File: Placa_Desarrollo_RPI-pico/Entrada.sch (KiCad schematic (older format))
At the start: 24 parts, among them J10 Conn_01x03_Female, J11 Conn_01x03_Female, J9 Conn_01x03_Female, SW2 SW_Push, SW3 Rotary_Encoder_Switch, SW4 SW_Push, SW5 SW_Push

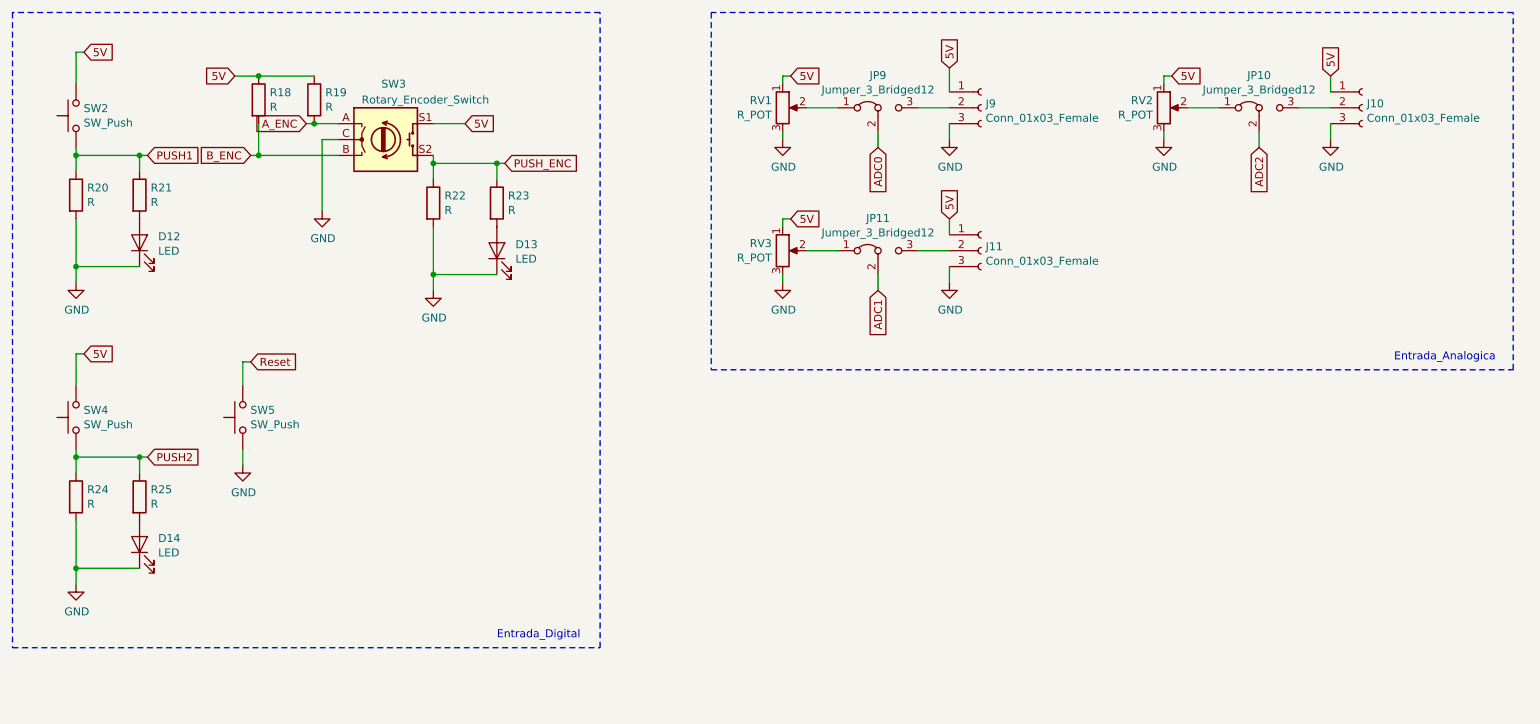
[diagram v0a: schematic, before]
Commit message: -
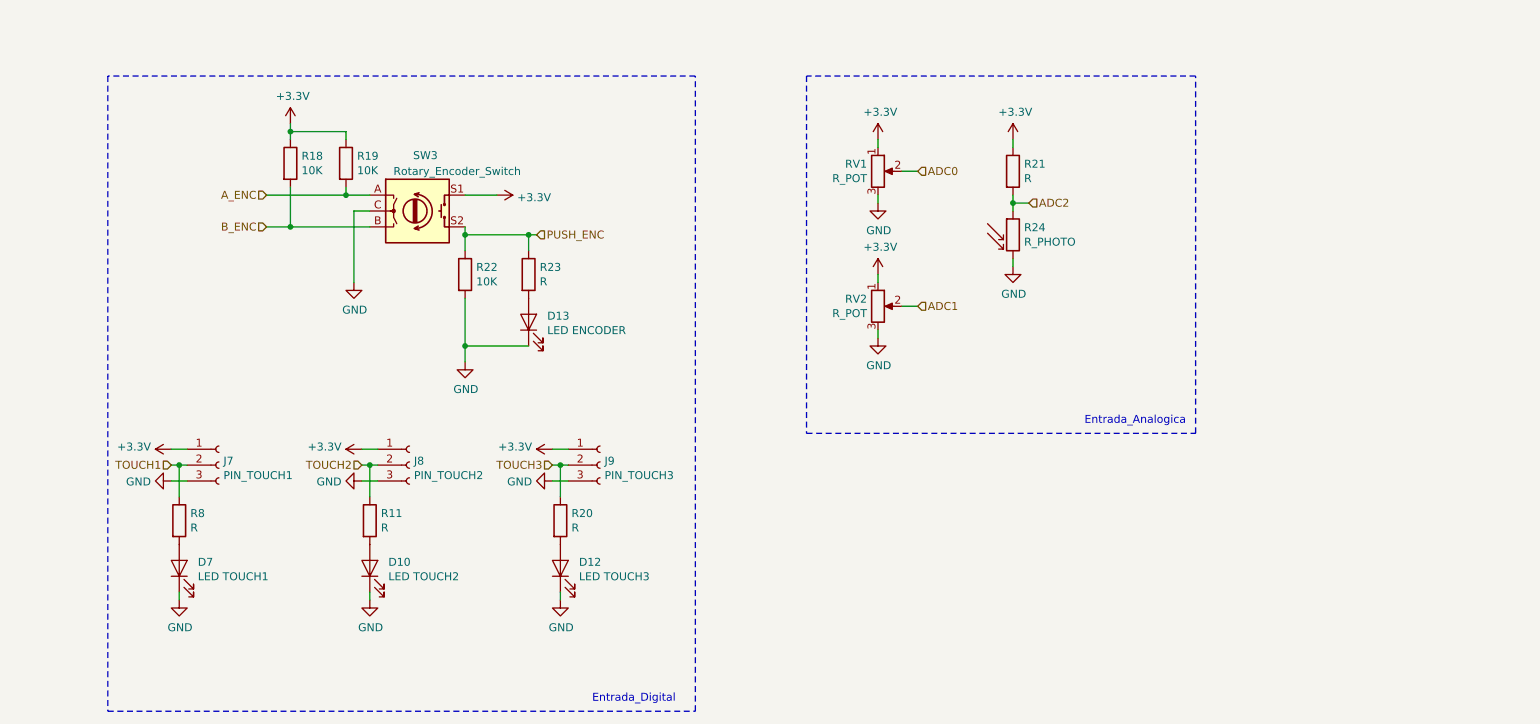
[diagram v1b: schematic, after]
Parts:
- removed D14: LED, symbol Device:LED
- removed J10, J11: Conn_01x03_Female, symbol Connector:Conn_01x03_Female
- removed JP10, JP11, JP9: Jumper_3_Bridged12, symbol Jumper:Jumper_3_Bridged12
- removed R24, R25: R, symbol Device:R
- removed RV3: R_POT, symbol Device:R_POT
- removed SW2, SW4, SW5: SW_Push, symbol Switch:SW_Push
- added D10: LED TOUCH2, symbol Device:LED
- added D7: LED TOUCH1, symbol Device:LED
- added J7: PIN_TOUCH1, symbol Connector:Conn_01x03_Female
- added J8: PIN_TOUCH2, symbol Connector:Conn_01x03_Female
- added R11, R8: R, symbol Device:R
- added R24: R_PHOTO, symbol Device:R_PHOTO
- D12: value LED -> LED TOUCH3
- D13: value LED -> LED ENCODER
- J9: value Conn_01x03_Female -> PIN_TOUCH3
- R18, R19, R22: value R -> 10K
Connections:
- net ADC0: now also RV1.2
- net ADC1: now also RV2.2
- net ADC2: now also R21.2, R24.1
- net GND: now also D10.1 (K), D7.1 (K), J7.3 (Pin_3), J8.3 (Pin_3), R24.2; no longer R20.2
- net at D12.2 (A): now also R20.2; no longer R21.2
- net TOUCH3: now reaches J9.2 (Pin_2)
- net TOUCH3: now also R20.1
- net 5V renamed +3V3
- net +3V3: now also R21.1, J7.1 (Pin_1), J8.1 (Pin_1)
- removed net PUSH1: R20.1, R21.1
- new net: D7.2 (A), R8.2
- new net: D10.2 (A), R11.2
- new net TOUCH1: J7.2 (Pin_2), R8.1
- new net TOUCH2: J8.2 (Pin_2), R11.1
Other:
- moved on the sheet: D13, R18, R19, R22, R23, RV1, SW3
